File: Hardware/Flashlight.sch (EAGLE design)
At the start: 13 parts

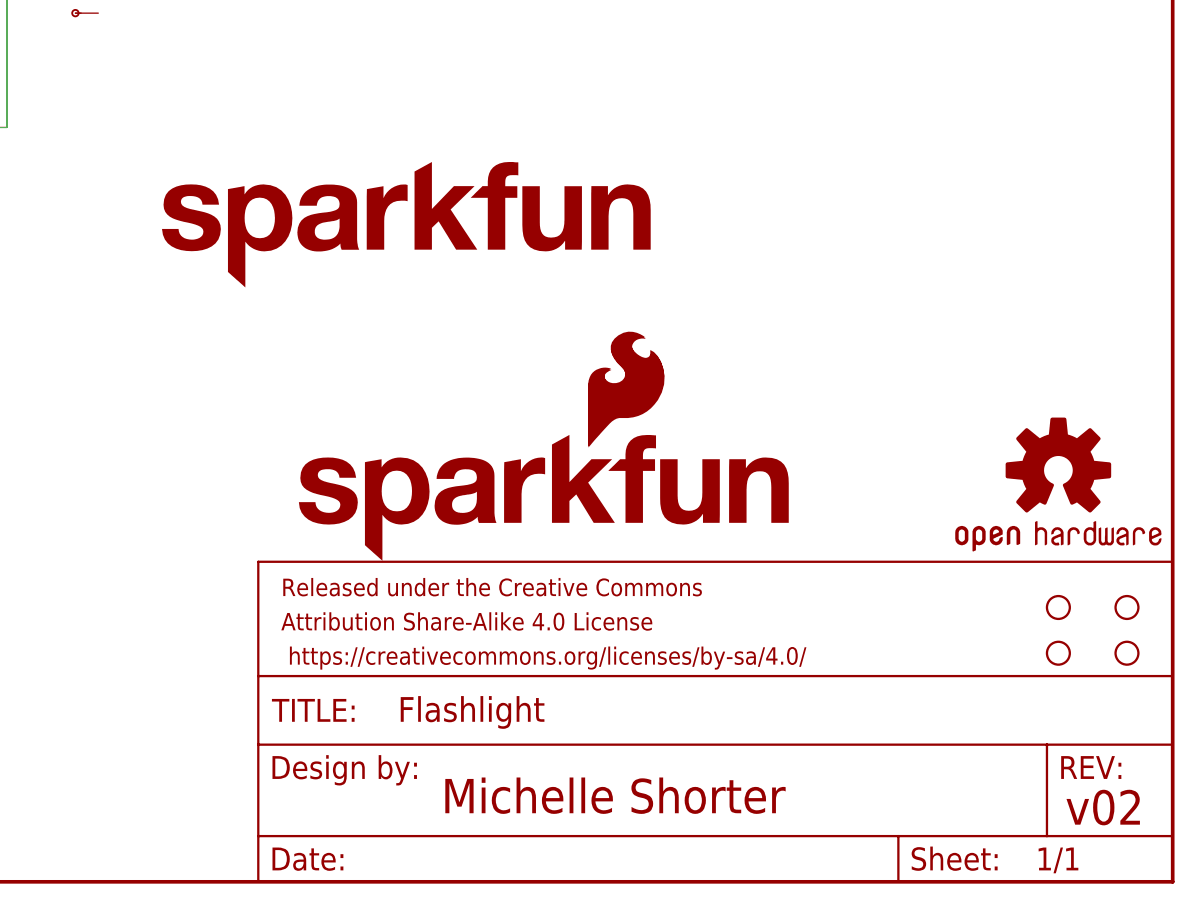
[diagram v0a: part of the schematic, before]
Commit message: V10
Updated version number on schematic, added library with Buzzard generated silk.  Removed gerber proto files and switch folder
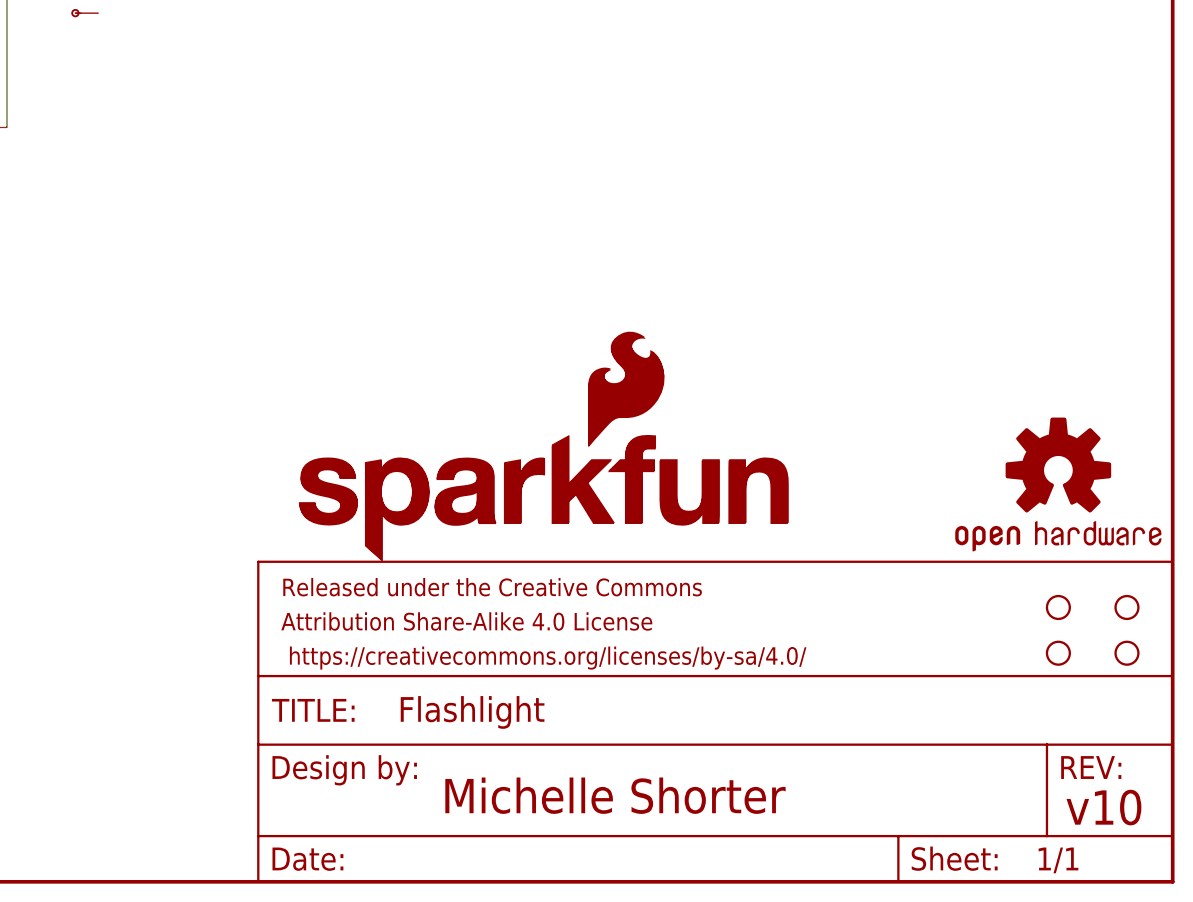
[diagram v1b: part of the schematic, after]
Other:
- note added: "v10"
- note removed: "v02"
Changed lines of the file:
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@@
 your circuit
 CR2032 - 3.0V</text>
-<text x="236.982" y="6.35" size="3.81" layer="94">v02</text>
+<text x="236.982" y="6.35" size="3.81" layer="94">v10</text>
 </plain>
 <instances>
@@
 <instance part="H3" gate="G$1" x="236.22" y="30.48"/>
 <instance part="H4" gate="G$1" x="243.84" y="30.48"/>
-<instance part="LOGO4" gate="G$1" x="134.62" y="66.04"/>
+<instance part="LOGO4" gate="G$1" x="149.86" y="35.56"/>
 </instances>
 <busses>
